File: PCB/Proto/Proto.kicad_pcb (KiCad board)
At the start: 2 copper layers, 102 x 102 mm, 88 parts, among them J1 Conn_01x40, J10 Conn_01x40, J11 Conn_01x40, J12 Conn_01x40, J13 Conn_01x40, J14 Conn_01x40, J15 Conn_01x40, J16 Conn_01x40, J17 Conn_01x40, J18 Conn_01x40, J19 Conn_01x40, J2 Conn_01x40, J20 Conn_01x40, J3 Conn_01x40, J4 Conn_01x40, J5 Conn_01x40, J6 Conn_01x40, J7 Conn_01x40, J8 Conn_01x40, J9 Conn_01x40

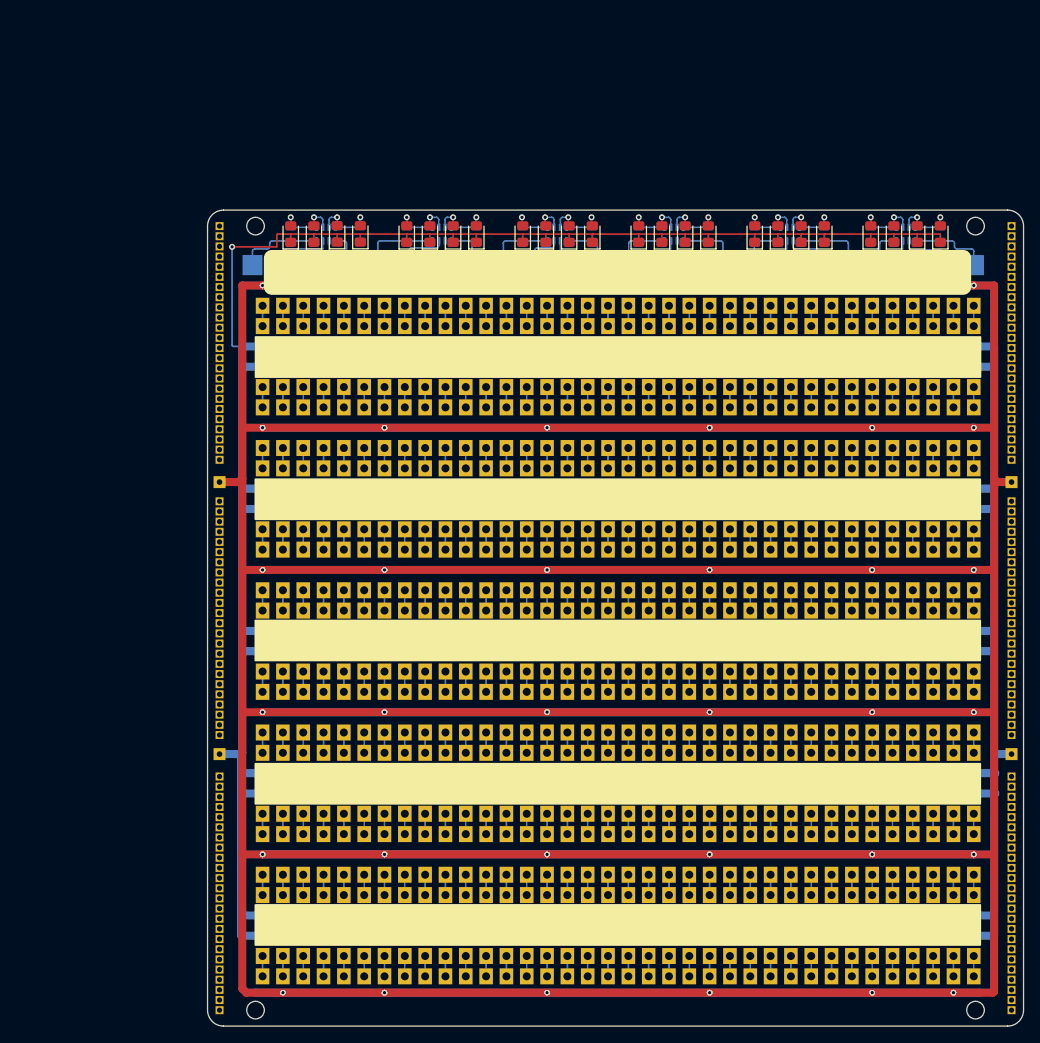
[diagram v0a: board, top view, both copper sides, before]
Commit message: WIP
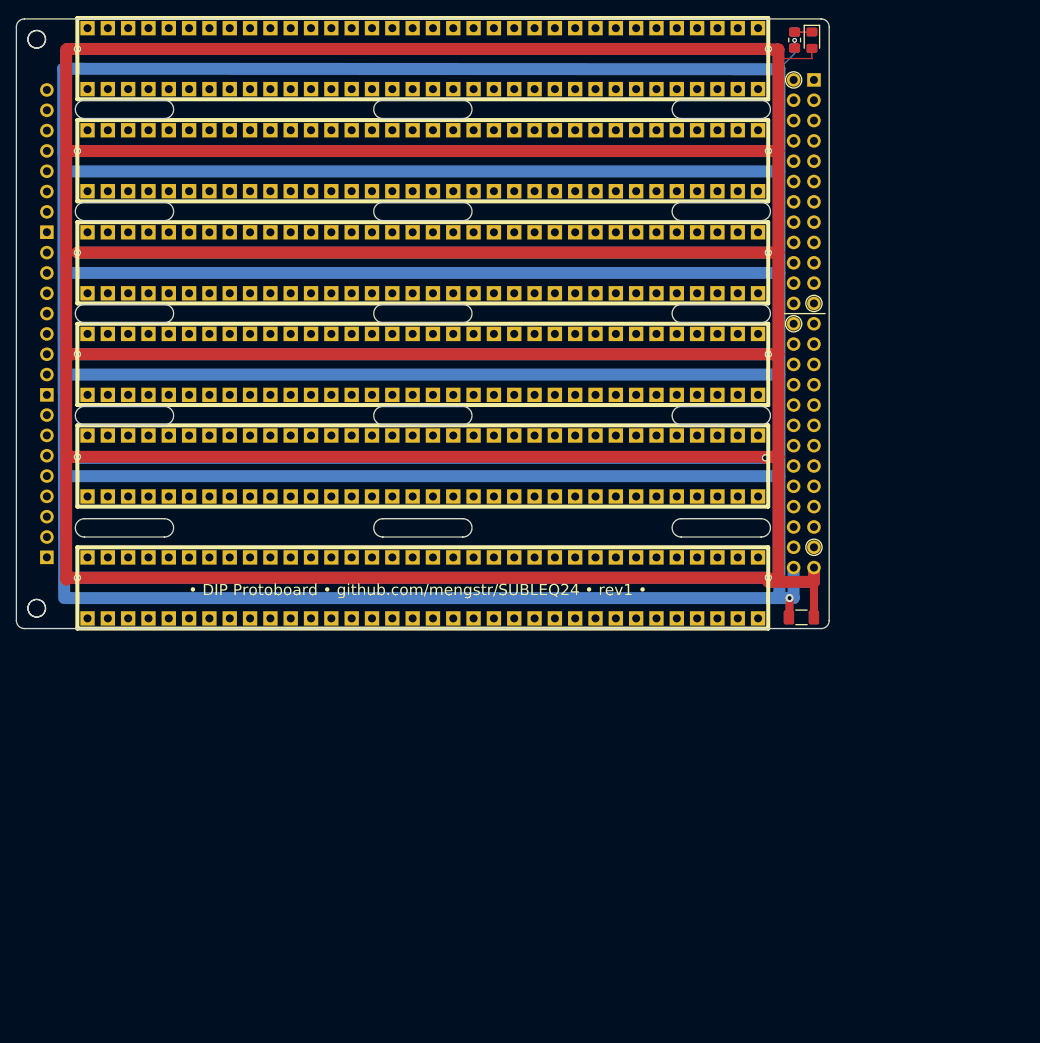
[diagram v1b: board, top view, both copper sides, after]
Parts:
- removed D1, D10, D11, D12, D13, D14, D15, D16, D17, D18, D19, D2, D20, D21, D22, D23, D24, D3, D4, D5, D6, D7, D8, D9: LED, LED_SMD:LED_0805_2012Metric_Pad1.15x1.40mm_HandSolder
- removed H1, H2: MountingHole, matseng:MountingHole_M2
- removed the H3 at (145.0, 51.0)
- removed the H4 at (55.0, 51.0)
- removed J1, J10, J11, J12, J13, J14, J15, J16, J17, J18, J19, J2, J20, J3, J5, J6, J7, J8, J9: Conn_01x40, matseng:PinSocket_1x36_P2.54mm_SQ_NoSilk
- removed the J4 at (55.9, 132.1)
- removed JBL1, JBR1, JML1, JMR1, JTL1, JTR1: Conn_01x24, matseng:PinHeader_1x24_P1.27mm_NoSilk
- removed RN1, RN2, RN3, RN4, RN5, RN6: R_Pack04, Resistor_SMD:R_Array_Concave_4x0603
- removed TP1, TP2, TP3, TP4: TestPoint, TestPoint:TestPoint_THTPad_1.5x1.5mm_Drill0.7mm
- removed TP10, TP11, TP12, TP13, TP14, TP15, TP16, TP17, TP18, TP19, TP20, TP21, TP22, TP23, TP24, TP25, TP26, TP27, TP28, TP5, TP6, TP7, TP8, TP9: TestPoint, TestPoint:TestPoint_Pad_2.5x2.5mm
- added BUS2: Conn_02x25_Odd_Even, Connector_PinHeader_2.54mm:PinHeader_2x25_P2.54mm_Vertical, B.Cu at (124.8, 32.7)
- added C96: C, Capacitor_SMD:C_1206_3216Metric_Pad1.33x1.80mm_HandSolder, F.Cu at (123.2, 99.9)
- added D97: LED, LED_SMD:LED_0805_2012Metric_Pad1.15x1.40mm_HandSolder, F.Cu at (124.5, 27.8)
- added H3, H4: MountingHole, matseng:MountingHole_M2, F.Cu at (27.6, 27.6)
- added H3, H4: MountingHole, matseng:MountingHole_M2, F.Cu at (27.6, 98.8)
- added J4: Conn_01x08_Pin, Connector_PinHeader_2.54mm:PinHeader_1x08_P2.54mm_Vertical, B.Cu at (28.9, 72.1)
- added J4: Conn_01x08_Pin, Connector_PinHeader_2.54mm:PinHeader_1x08_P2.54mm_Vertical, B.Cu at (28.9, 92.4)
- added J4: Conn_01x08_Pin, Connector_PinHeader_2.54mm:PinHeader_1x08_P2.54mm_Vertical, B.Cu at (28.9, 51.8)
- added R98: R, Resistor_SMD:R_0805_2012Metric_Pad1.20x1.40mm_HandSolder, F.Cu at (122.4, 27.7)
- added REF**: PinHeader_1x34_P2.54mm_Vertical, Connector_PinHeader_2.54mm:PinHeader_1x34_P2.54mm_Vertical, F.Cu at (34.0, 100.0)
- added REF**: PinHeader_1x34_P2.54mm_Vertical, Connector_PinHeader_2.54mm:PinHeader_1x34_P2.54mm_Vertical, F.Cu at (34.0, 72.1)
- added REF**: PinHeader_1x34_P2.54mm_Vertical, Connector_PinHeader_2.54mm:PinHeader_1x34_P2.54mm_Vertical, F.Cu at (34.0, 26.3)
- added REF**: PinHeader_1x34_P2.54mm_Vertical, Connector_PinHeader_2.54mm:PinHeader_1x34_P2.54mm_Vertical, F.Cu at (34.0, 77.2)
- added REF**: PinHeader_1x34_P2.54mm_Vertical, Connector_PinHeader_2.54mm:PinHeader_1x34_P2.54mm_Vertical, F.Cu at (34.0, 64.5)
- added REF**: PinHeader_1x34_P2.54mm_Vertical, Connector_PinHeader_2.54mm:PinHeader_1x34_P2.54mm_Vertical, F.Cu at (34.0, 92.4)
- added REF**: PinHeader_1x34_P2.54mm_Vertical, Connector_PinHeader_2.54mm:PinHeader_1x34_P2.54mm_Vertical, F.Cu at (34.0, 39.0)
- added REF**: PinHeader_1x34_P2.54mm_Vertical, Connector_PinHeader_2.54mm:PinHeader_1x34_P2.54mm_Vertical, F.Cu at (34.0, 84.8)
- added REF**: PinHeader_1x34_P2.54mm_Vertical, Connector_PinHeader_2.54mm:PinHeader_1x34_P2.54mm_Vertical, F.Cu at (34.0, 59.4)
- added REF**: PinHeader_1x34_P2.54mm_Vertical, Connector_PinHeader_2.54mm:PinHeader_1x34_P2.54mm_Vertical, F.Cu at (34.0, 51.8)
- added REF**: PinHeader_1x34_P2.54mm_Vertical, Connector_PinHeader_2.54mm:PinHeader_1x34_P2.54mm_Vertical, F.Cu at (34.0, 33.9)
- added REF**: PinHeader_1x34_P2.54mm_Vertical, Connector_PinHeader_2.54mm:PinHeader_1x34_P2.54mm_Vertical, F.Cu at (34.0, 46.6)
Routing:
- net (no net): track 0.00 -> 1721.6 mm, vias 0 -> 14
- net VCC: track 1280.8 -> 0.00 mm, vias 36 -> 0
- net GNDD: track 1221.0 -> 0.00 mm, vias 1 -> 0
- net Net-(RN1-R4.1): track 10.3 -> 0.00 mm
- net Net-(RN6-R1.1): track 9.64 -> 0.00 mm
- net Net-(RN2-R4.1): track 9.45 -> 0.00 mm
- net Net-(RN5-R1.1): track 8.74 -> 0.00 mm
- net Net-(RN3-R4.1): track 8.17 -> 0.00 mm
- net Net-(RN4-R1.1): track 7.56 -> 0.00 mm
- net Net-(RN1-R3.1): track 7.49 -> 0.00 mm
- net Net-(RN4-R4.1): track 7.08 -> 0.00 mm
- net Net-(RN6-R2.1): track 6.66 -> 0.00 mm
- net Net-(RN3-R1.1): track 6.47 -> 0.00 mm
- net Net-(RN2-R3.1): track 6.19 -> 0.00 mm
- net Net-(RN5-R4.1): track 5.90 -> 0.00 mm
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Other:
- board size 102 x 102 mm -> 101.6 x 76.2 mm
- board text added: "• DIP Protoboard • github.com/mengstr/SUBLEQ24 • rev1 •"
- board text removed: "19 OCTOBER 2003"
- board text removed: "DISCRETE 24 BIT SUBLEQ"
- board text removed: "GITHUB.COM/MENGSTR/SUBLEQ24"
- board text removed: "PROTOBOARD"
